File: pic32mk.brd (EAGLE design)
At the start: 110.2 x 85.1 mm, 92 parts, among them IC1 PIC32MK1024MCF100-I_PT, IC10 5.0VDC, IC11 3.3VDC, IC2 ADM3095EBRZ, IC3 TXB0101DCKR, IC4 MAX203ECWP, IC5 TXB0101DCKR, IC6 TXB0101DCKR, IC7 TXB0101DCKR, IC8 TXB0101DCKR, IC9 TXB0101DCKR, J1 1-1586043-4, U1 PMIC-MC33932VW(SOP44), U2 PMIC-MC33932VW(SOP44), U3 ULN2803ADW, U4 REF3440IDBVR, X1 22-23-2101, X2 22-23-2081, X3 53261-10

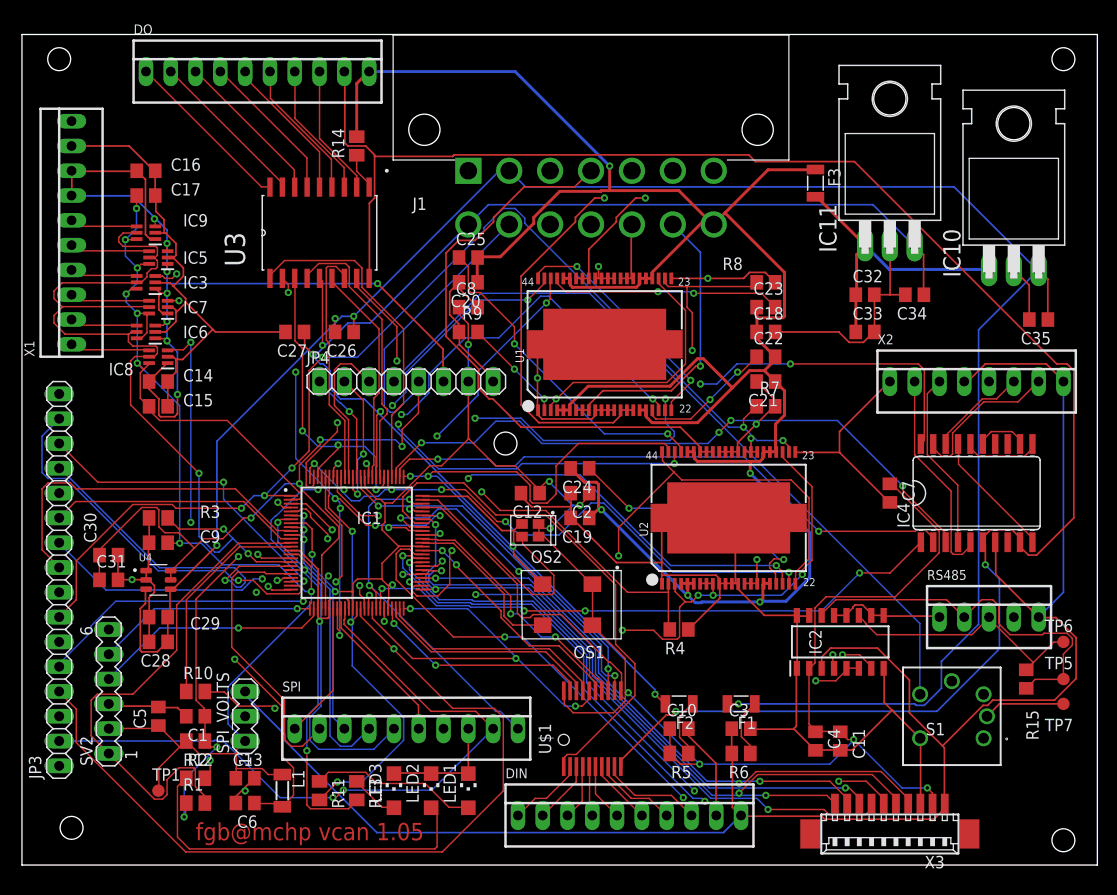
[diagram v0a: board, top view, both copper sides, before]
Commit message: up
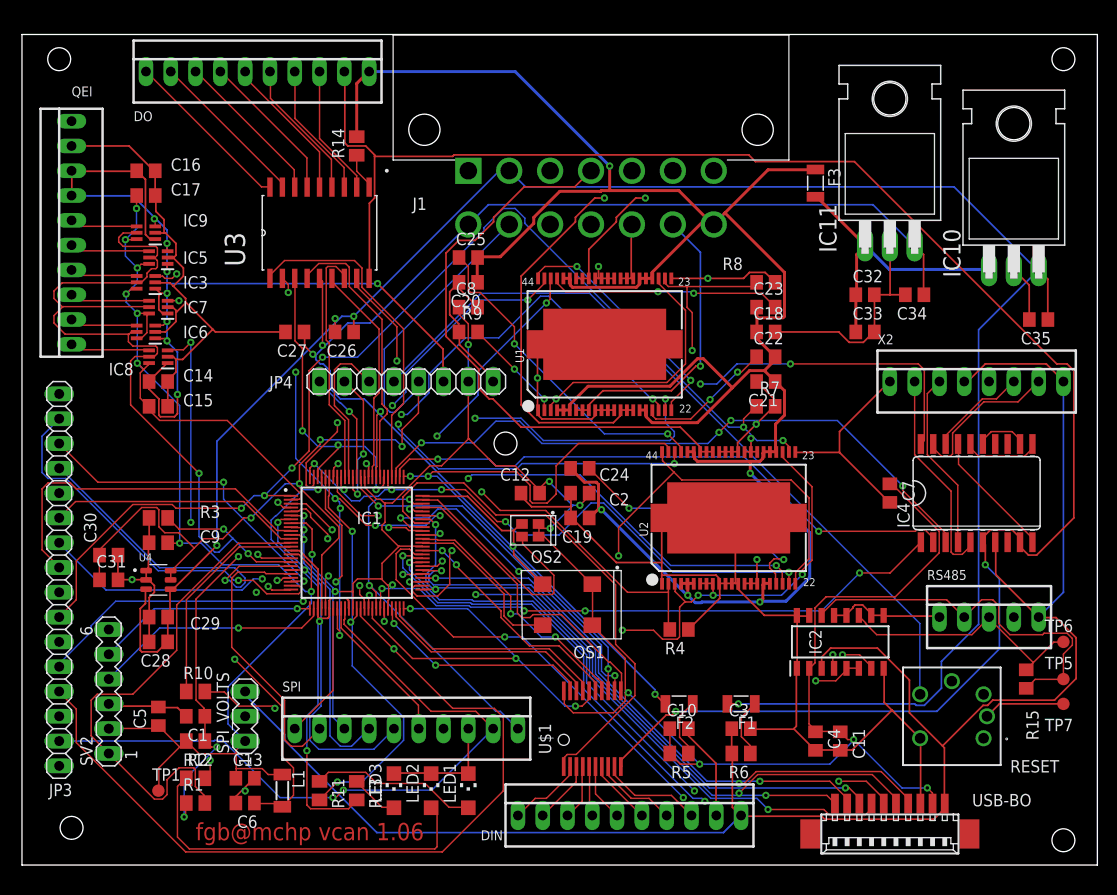
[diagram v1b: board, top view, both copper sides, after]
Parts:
- renumbered S1 to RESET, X1 to QEI, X3 to USB-BO
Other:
- board text added: "fgb@mchp vcan 1.06"
- board text removed: "fgb@mchp vcan 1.05"
